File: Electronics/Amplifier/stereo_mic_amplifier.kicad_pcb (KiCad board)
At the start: 2 copper layers, 34.2 x 45.3 mm, 26 parts, among them P1 mic_L, P2 mic_R, P3 batt, P4 CONN_01X03, U1 TL072

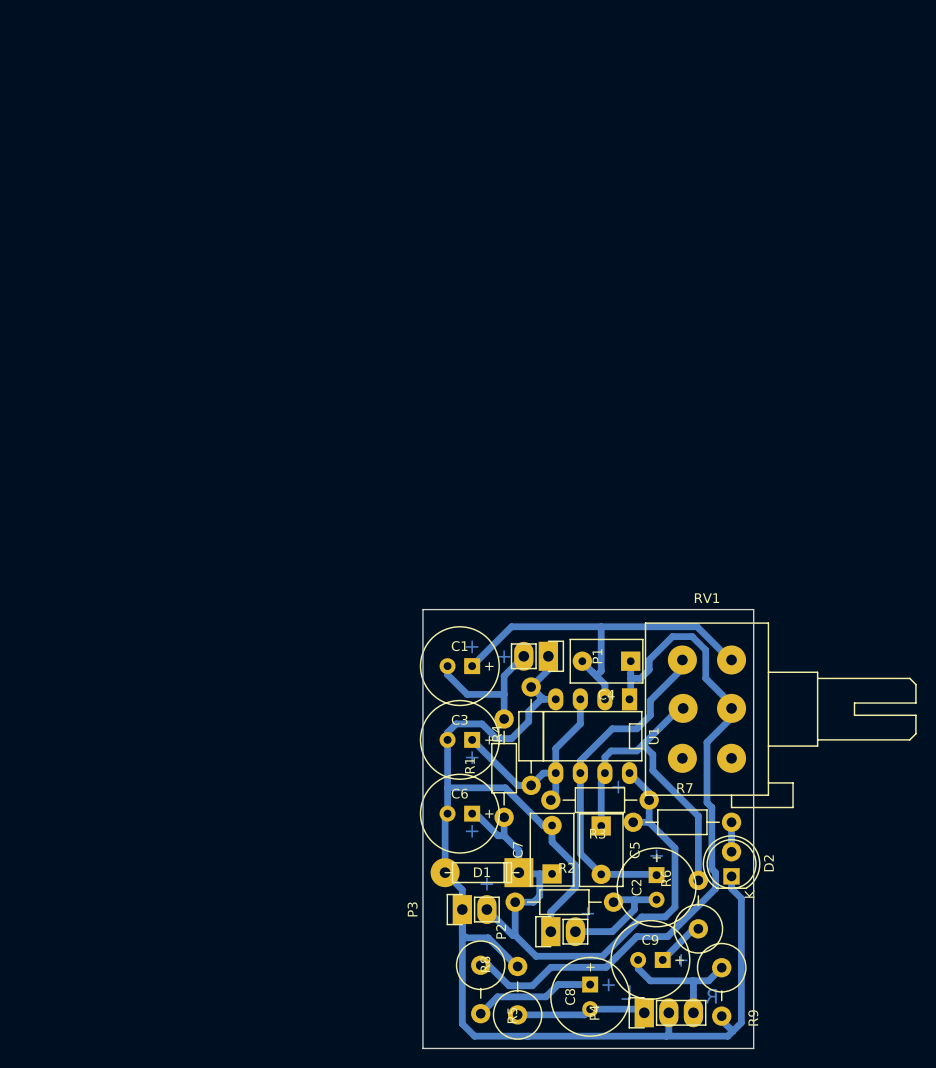
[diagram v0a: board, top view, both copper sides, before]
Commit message: Updated layout & cnc files
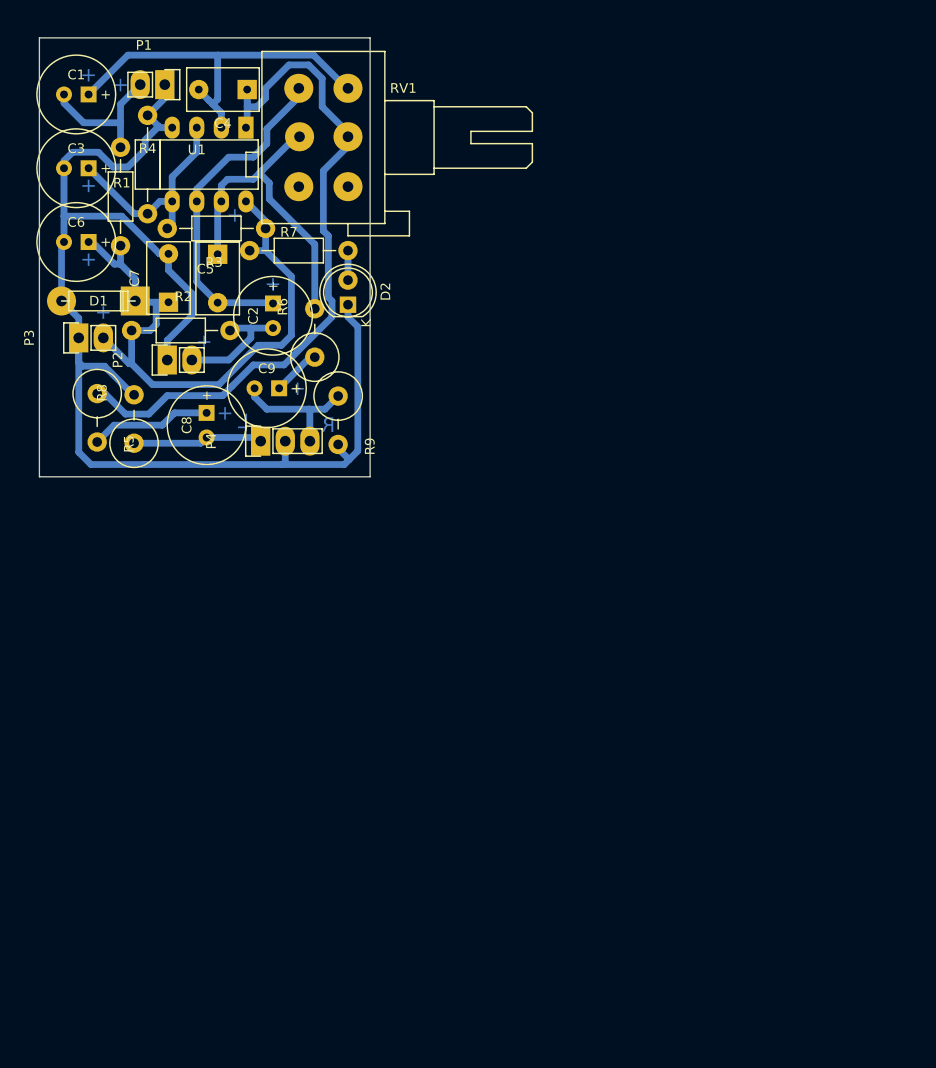
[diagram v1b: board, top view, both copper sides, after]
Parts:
- moved C1 71.1 mm to (37.7, 35.7)
- moved C2 71.1 mm to (58.0, 58.5)
- moved C6 71.1 mm to (37.7, 50.9)
- moved C7 71.1 mm to (47.2, 57.1)
- moved C8 71.1 mm to (51.2, 69.8)
- moved D1 71.1 mm to (40.0, 57.0)
- moved D2 71.1 mm to (65.8, 57.4)
- moved P1 71.1 mm to (46.9, 34.7)
- moved P2 71.1 mm to (47.1, 63.1)
- moved P3 71.1 mm to (38.0, 60.8)
- moved P4 71.1 mm to (56.8, 71.5)
- moved R1 71.1 mm to (42.3, 46.2)
- moved R2 71.1 mm to (48.5, 60.1)
- moved R5 71.1 mm to (39.9, 69.1)
- moved R8 71.1 mm to (43.7, 69.2)
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
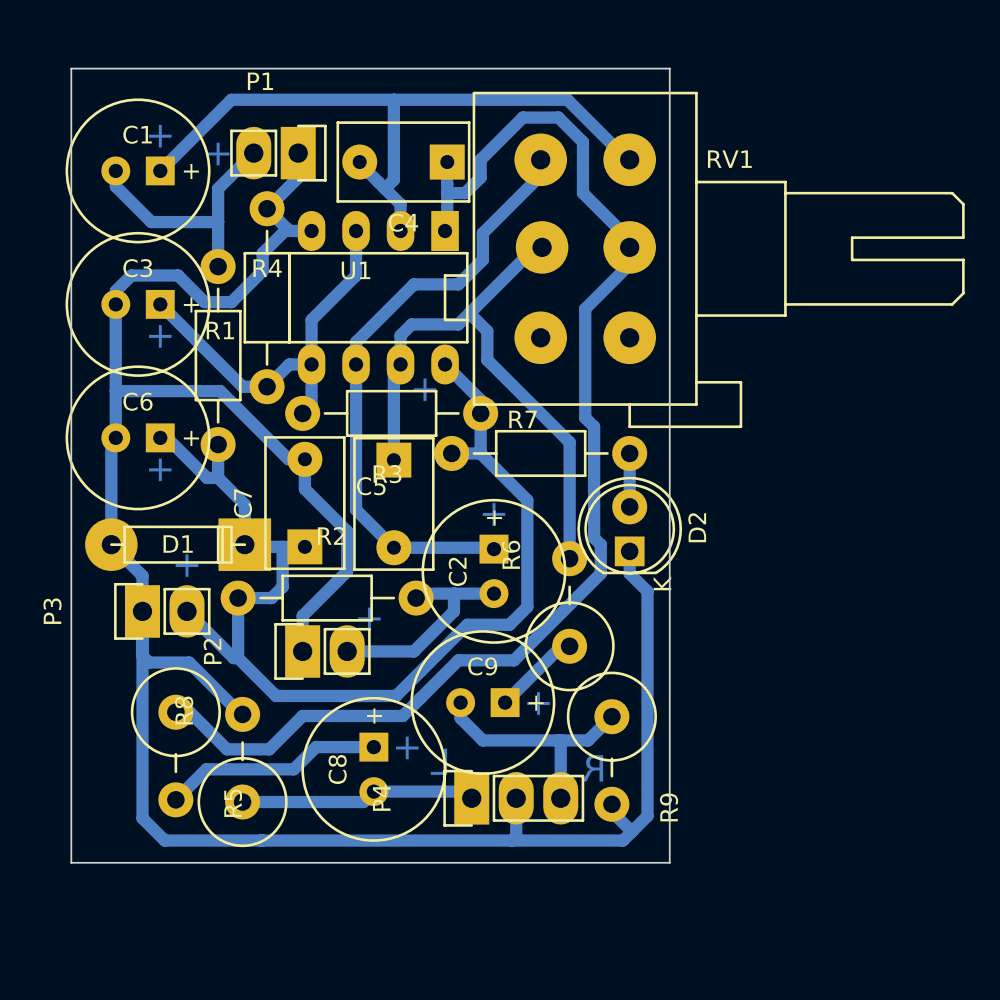
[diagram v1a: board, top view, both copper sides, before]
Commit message: rotated gerber
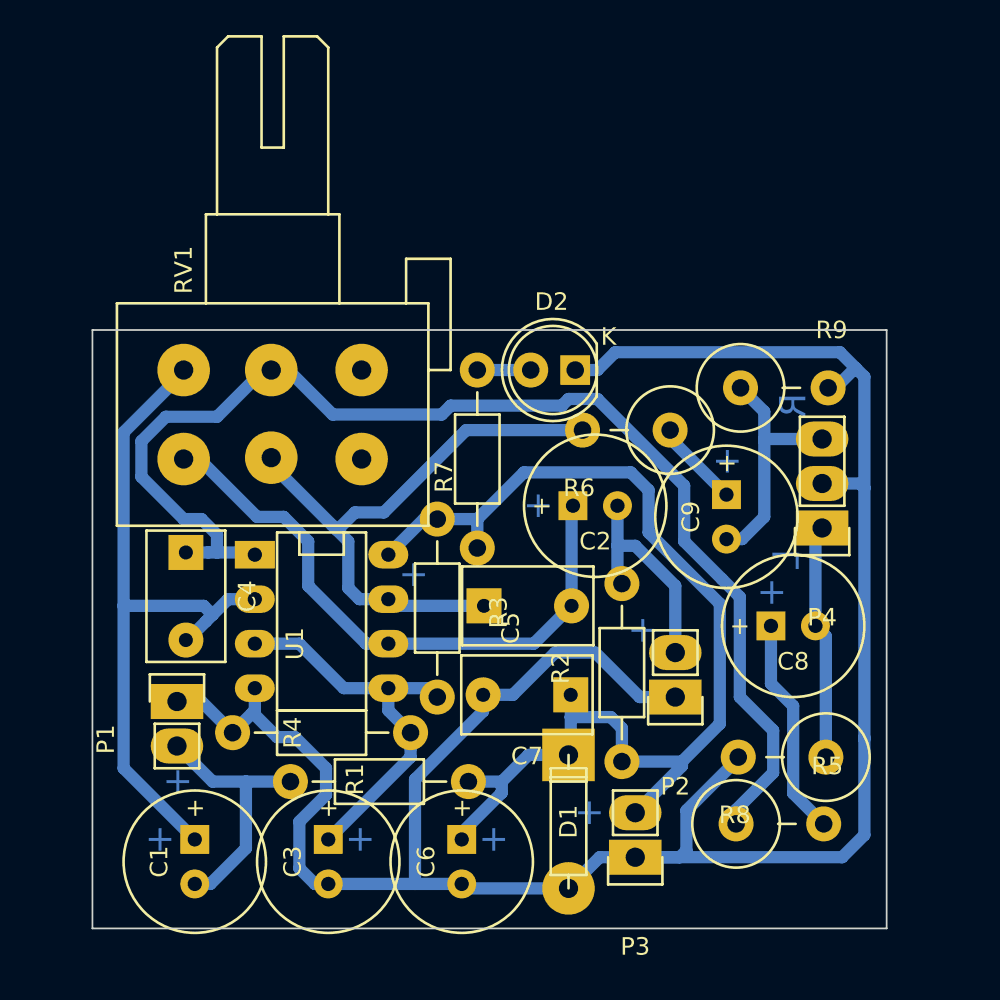
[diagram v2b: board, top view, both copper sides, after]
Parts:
- moved C1 39.6 mm to (41.0, 75.1), turned to 270 degrees
- moved R5 34.7 mm to (74.4, 73.0), turned to 0 degrees
- moved C3 33.6 mm to (48.6, 75.1), turned to 270 degrees
- moved P1 32.1 mm to (39.9, 66.0), turned to 0 degrees
- moved P3 31.4 mm to (66.1, 74.9), turned to 180 degrees
- moved R8 30.8 mm to (74.5, 69.2), turned to 180 degrees
- moved C6 30.4 mm to (56.2, 75.1), turned to 270 degrees
- moved D1 27.3 mm to (62.3, 72.8), turned to 90 degrees
- moved C4 26.8 mm to (40.4, 57.5), turned to 270 degrees
- moved R1 26.0 mm to (51.5, 70.5), turned to 180 degrees
- moved C8 25.3 mm to (75.1, 61.7), turned to 0 degrees
- moved P4 25.3 mm to (76.8, 56.1), turned to 180 degrees
- moved R4 25.0 mm to (48.2, 67.8), turned to 180 degrees
- moved R9 23.4 mm to (74.6, 48.1), turned to 0 degrees
- moved P2 21.4 mm to (68.4, 65.7), turned to 180 degrees
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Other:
- board size 34.2 x 45.3 mm -> 45.3 x 34.2 mm
